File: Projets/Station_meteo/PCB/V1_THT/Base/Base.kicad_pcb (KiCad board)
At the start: 2 copper layers, 232.8 x 97.6 mm, 65 parts, among them J1 Conn_02x05_Odd_Even, J13 JST_Connector, J15 SolderJumper_2_Bridged, J16 SolderJumper_2_Bridged, J2 Conn_02x04_Odd_Even, J3 Conn_02x06_Odd_Even, J4 Conn_02x06_Odd_Even, J5 Screw_Terminal_01x02_2.54mm, J6 Conn_01x03_Pin, J7 USR_BTN, J8 USB_C_Receptacle, Q1 FDS4559, Q2 2N7002H, Q3 FDS4559, Q4 2N7002H, SW1 SW_B, T10 TP, T11 TP, T9 TP, U1 ATmega328P-P, U10 CH340G, U3 DS3231M, U4 LM358, U5 74HC123, U6 AMS1117-3.3, U7 NRF24L01_Breakout, Y1 Crystal, Y2 12MHz

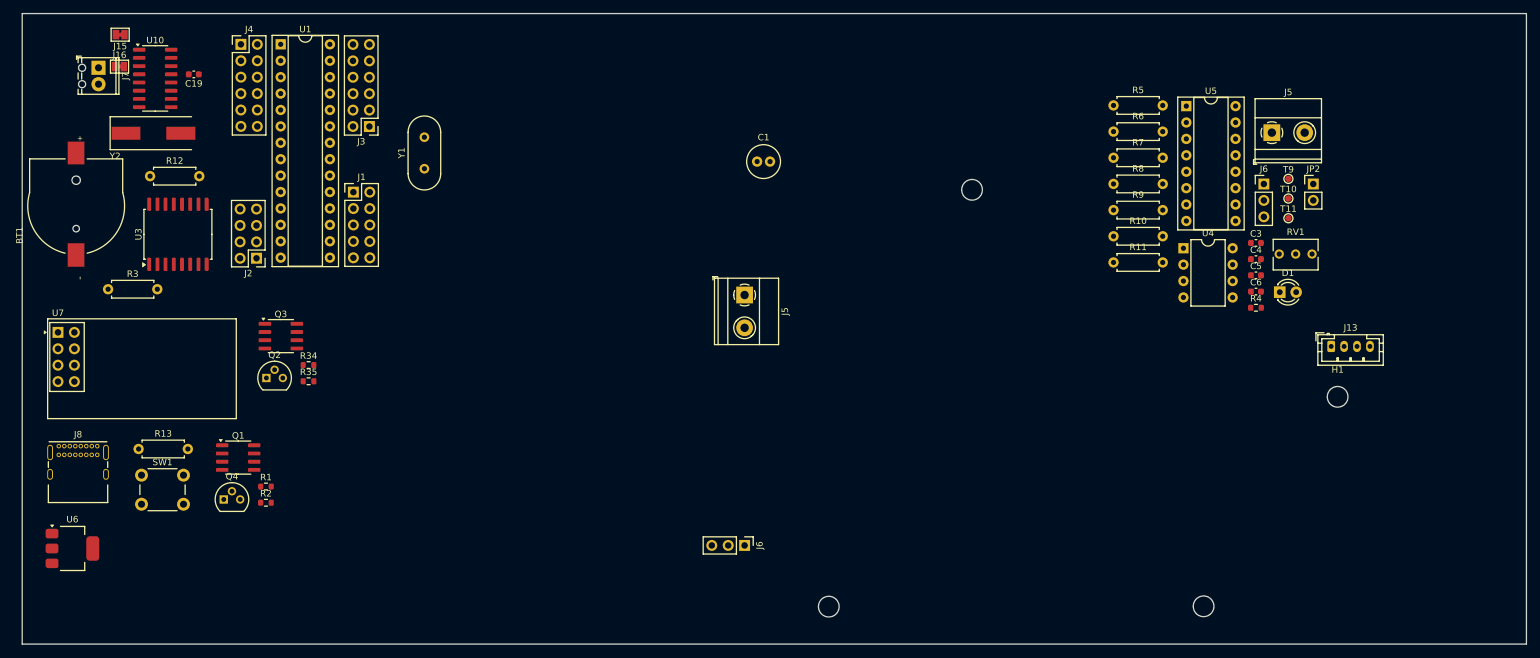
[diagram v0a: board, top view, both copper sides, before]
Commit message: Update Weather station
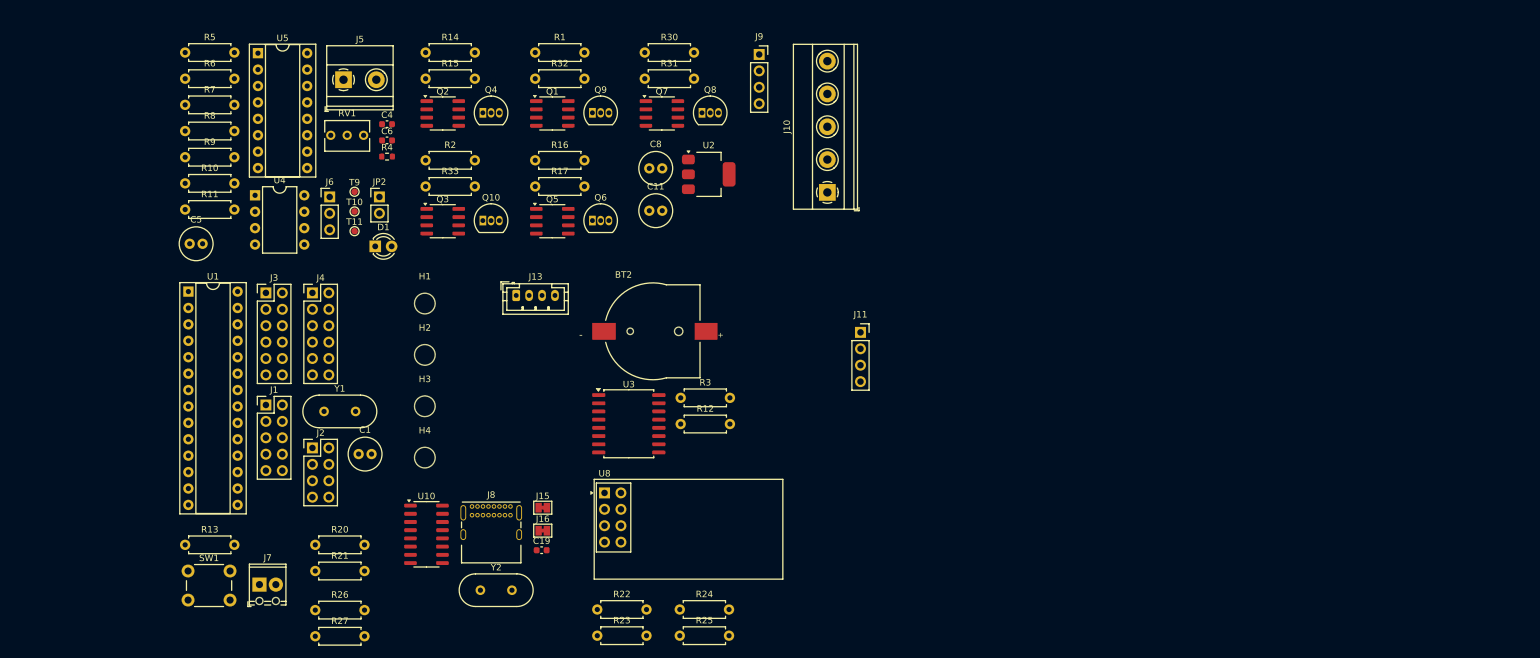
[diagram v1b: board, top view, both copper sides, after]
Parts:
- removed BT1: Battery_Cell, CREPP_Batteries_holders:MPD_BC501SM-TR
- removed C3: 100nF, Capacitor_SMD:C_0603_1608Metric
- removed the J5 at (175.3, 77.8)
- removed the J5 at (256.9, 52.7)
- removed the J6 at (255.7, 60.6)
- removed the J6 at (175.3, 116.6)
- removed R34: 10k, Resistor_SMD:R_0603_1608Metric
- removed R35: 100k, Resistor_SMD:R_0603_1608Metric
- removed the S1 at (246.2, 38.8)
- removed the S1 at (259.6, 86.6)
- removed U6: AMS1117-3.3, Package_TO_SOT_SMD:SOT-223-3_TabPin2
- removed U7: NRF24L01_Breakout, RF_Module:nRF24L01_Breakout
- added BT2: Battery_Cell, CREPP_Batteries_holders:MPD_BC501SM-TR, F.Cu at (161.1, 83.4)
- added C11: 10uF, Capacitor_THT:C_Radial_D5.0mm_H11.0mm_P2.00mm, F.Cu at (160.6, 64.7)
- added C8: 10uF, Capacitor_THT:C_Radial_D5.0mm_H11.0mm_P2.00mm, F.Cu at (160.6, 58.2)
- added J10: Screw_Terminal_01x05_5.08mm, TerminalBlock_Phoenix:TerminalBlock_Phoenix_MKDS-1,5-5-5.08_1x05_P5.08mm_Horizontal, F.Cu at (188.2, 61.9)
- added J11: GNSS_Virtual, Connector_PinSocket_2.54mm:PinSocket_1x04_P2.54mm_Vertical, F.Cu at (193.3, 83.6)
- added J5: Screw_Terminal_01x02_2.54mm, TerminalBlock_Phoenix:TerminalBlock_Phoenix_MKDS-1,5-2-5.08_1x02_P5.08mm_Horizontal, F.Cu at (113.3, 44.5)
- added J6: Conn_01x03_Pin, Connector_PinHeader_2.54mm:PinHeader_1x03_P2.54mm_Vertical, F.Cu at (111.1, 62.6)
- added J9: Conn_01x04_Socket, Connector_PinSocket_2.54mm:PinSocket_1x04_P2.54mm_Vertical, F.Cu at (177.6, 40.6)
- added Q10: 2N7000, Package_TO_SOT_THT:TO-92_Inline, F.Cu at (134.8, 66.3)
- added Q5: FDS4559, Package_SO:SOIC-8_3.9x4.9mm_P1.27mm, F.Cu at (145.6, 66.4)
- added Q6: 2N7000, Package_TO_SOT_THT:TO-92_Inline, F.Cu at (151.8, 66.3)
- added Q7: FDS4559, Package_SO:SOIC-8_3.9x4.9mm_P1.27mm, F.Cu at (162.5, 49.7)
- added Q8: 2N7000, Package_TO_SOT_THT:TO-92_Inline, F.Cu at (168.7, 49.6)
- added Q9: 2N7000, Package_TO_SOT_THT:TO-92_Inline, F.Cu at (151.8, 49.6)
- added R14: 10k, Resistor_THT:R_Axial_DIN0207_L6.3mm_D2.5mm_P7.62mm_Horizontal, F.Cu at (126.0, 40.3)
- added R15: 10k, Resistor_THT:R_Axial_DIN0207_L6.3mm_D2.5mm_P7.62mm_Horizontal, F.Cu at (126.0, 44.3)
- added R16: 10k, Resistor_THT:R_Axial_DIN0207_L6.3mm_D2.5mm_P7.62mm_Horizontal, F.Cu at (142.9, 56.9)
- added R17: 10k, Resistor_THT:R_Axial_DIN0207_L6.3mm_D2.5mm_P7.62mm_Horizontal, F.Cu at (142.9, 61.0)
- added R20: 10k, Resistor_THT:R_Axial_DIN0207_L6.3mm_D2.5mm_P7.62mm_Horizontal, F.Cu at (108.9, 116.5)
- added R21: 10k, Resistor_THT:R_Axial_DIN0207_L6.3mm_D2.5mm_P7.62mm_Horizontal, F.Cu at (108.9, 120.5)
- added R22: 10k, Resistor_THT:R_Axial_DIN0207_L6.3mm_D2.5mm_P7.62mm_Horizontal, F.Cu at (152.5, 126.5)
- added R23: 10k, Resistor_THT:R_Axial_DIN0207_L6.3mm_D2.5mm_P7.62mm_Horizontal, F.Cu at (152.5, 130.5)
- added R24: 10k, Resistor_THT:R_Axial_DIN0207_L6.3mm_D2.5mm_P7.62mm_Horizontal, F.Cu at (165.3, 126.5)
- added R25: 10k, Resistor_THT:R_Axial_DIN0207_L6.3mm_D2.5mm_P7.62mm_Horizontal, F.Cu at (165.3, 130.5)
- added R26: 10k, Resistor_THT:R_Axial_DIN0207_L6.3mm_D2.5mm_P7.62mm_Horizontal, F.Cu at (108.9, 126.6)
- added R27: 10k, Resistor_THT:R_Axial_DIN0207_L6.3mm_D2.5mm_P7.62mm_Horizontal, F.Cu at (108.9, 130.6)
- added R30: 10k, Resistor_THT:R_Axial_DIN0207_L6.3mm_D2.5mm_P7.62mm_Horizontal, F.Cu at (159.9, 40.3)
- added R31: 10k, Resistor_THT:R_Axial_DIN0207_L6.3mm_D2.5mm_P7.62mm_Horizontal, F.Cu at (159.9, 44.3)
- added R32: 10k, Resistor_THT:R_Axial_DIN0207_L6.3mm_D2.5mm_P7.62mm_Horizontal, F.Cu at (142.9, 44.3)
- added R33: 10k, Resistor_THT:R_Axial_DIN0207_L6.3mm_D2.5mm_P7.62mm_Horizontal, F.Cu at (126.0, 61.0)
- added S1: ~, CREPP_Spacers:Spacer_M3_MF_05mm, F.Cu at (133.4, 78.7)
- added U2: AMS1117-3.3, Package_TO_SOT_SMD:SOT-223-3_TabPin2, F.Cu at (169.8, 59.1)
- added U8: NRF24L01_Breakout, RF_Module:nRF24L01_Breakout, F.Cu at (153.7, 108.4)
- C1: value 100nF -> 10uF
- C5: value 100nF -> 10uF; footprint Capacitor_SMD:C_0603_1608Metric -> Capacitor_THT:C_Radial_D5.0mm_H11.0mm_P2.00mm
- J13: value JST_Connector -> JST_PH_4P
- Q2: value 2N7002H -> FDS4559; footprint Package_TO_SOT_THT:TO-92 -> Package_SO:SOIC-8_3.9x4.9mm_P1.27mm
- Q4: value 2N7002H -> 2N7000; footprint Package_TO_SOT_THT:TO-92 -> Package_TO_SOT_THT:TO-92_Inline
- R1: footprint Resistor_SMD:R_0603_1608Metric -> Resistor_THT:R_Axial_DIN0207_L6.3mm_D2.5mm_P7.62mm_Horizontal
- R2: value 100k -> 10k; footprint Resistor_SMD:R_0603_1608Metric -> Resistor_THT:R_Axial_DIN0207_L6.3mm_D2.5mm_P7.62mm_Horizontal
- Y2: value 12MHz -> Crystal; footprint Crystal:Crystal_SMD_HC49-SD -> Crystal:Crystal_HC49-4H_Vertical
- moved C5 165.1 mm to (89.4, 69.9)
- moved RV1 147.9 mm to (116.4, 53.1)
- moved T10 144.6 mm to (115.0, 64.9)
- moved T11 144.6 mm to (115.0, 67.9)
- moved T9 144.6 mm to (115.0, 61.8)
- moved JP2 144.6 mm to (118.8, 62.6)
- moved U4 143.9 mm to (99.6, 62.4)
- moved U5 143.9 mm to (100.0, 40.4)
- moved R10 143.9 mm to (88.7, 60.5)
- moved R11 143.9 mm to (88.7, 64.6)
- moved R5 143.9 mm to (88.7, 40.3)
- moved R6 143.9 mm to (88.7, 44.3)
- moved R7 143.9 mm to (88.7, 48.4)
- moved R8 143.9 mm to (88.7, 52.4)
- moved R9 143.9 mm to (88.7, 56.5)
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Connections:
- C1 pad 1: GND -> /MCU/+VCC
- C1 pad 2: /MCU/+VCC -> GND
- J13 pad 1: /VCC -> /+5V
- J7 pad 1: /Reset/RESET -> /MCU/~{RESET}/PC6
- J7 pad 2: /Reset/GND -> GND
- Q1 pad 7: /Power_Handler_Anemo/V_{IN} -> /+5V
- Q1 pad 8: /Power_Handler_Anemo/V_{IN} -> /+5V
- Q2 pad 1: /Power_Handler_RTC/ENABLE -> /NRF24/+3.3V
- Q2 pad 2: GND -> Net-(Q2A-G)
- Q2 pad 3: Net-(Q2-D) -> (no net)
- Q3 pad 2: Net-(Q2-D) -> Net-(Q10-D)
- Q3 pad 7: /Power_Handler_RTC/V_{IN} -> /+5V
- Q3 pad 8: /Power_Handler_RTC/V_{IN} -> /+5V
- Q4 pad 1: /Power_Handler_Anemo/ENABLE -> GND
- Q4 pad 2: GND -> /Power_Handler_NRF24/ENABLE
- Q4 pad 3: Net-(Q1A-G) -> Net-(Q2A-G)
- R1 pad 2: /Power_Handler_Anemo/V_{IN} -> /+5V
- R13 pad 1: /Reset/VCC -> /+5V
- R13 pad 2: /Reset/RESET -> /MCU/~{RESET}/PC6
- R2 pad 1: /Power_Handler_Anemo/ENABLE -> Net-(Q10-D)
- R2 pad 2: GND -> /+5V
- SW1 pad 1: /Reset/GND -> GND
- SW1 pad 2: /Reset/RESET -> /MCU/~{RESET}/PC6
- Y2 pad 1: Net-(U10-XI) -> Net-(U10-XO)
- Y2 pad 2: Net-(U10-XO) -> Net-(U10-XI)
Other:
- board outline removed
